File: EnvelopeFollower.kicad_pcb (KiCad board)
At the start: 2 copper layers, 177.9 x 87.9 mm, 87 parts, among them J1 RTip, J10 IN, J11 GND, J12 GND, J13 SW1B, J14 OUT, J15 DTIP, J16 DSW, J17 GND, J18 ITIP, J19 ISLV, J20 SW1C, J3 +9v, J4 GND, J5 SEND, J6 RSLV, J7 GND, J8 GND, J9 SW1A, SW1 Moog, SW2 BANDWIDTH, SW3 MODE, U1 TL074, U2 LM1458, U3 VTL5C, U4 VTL5C

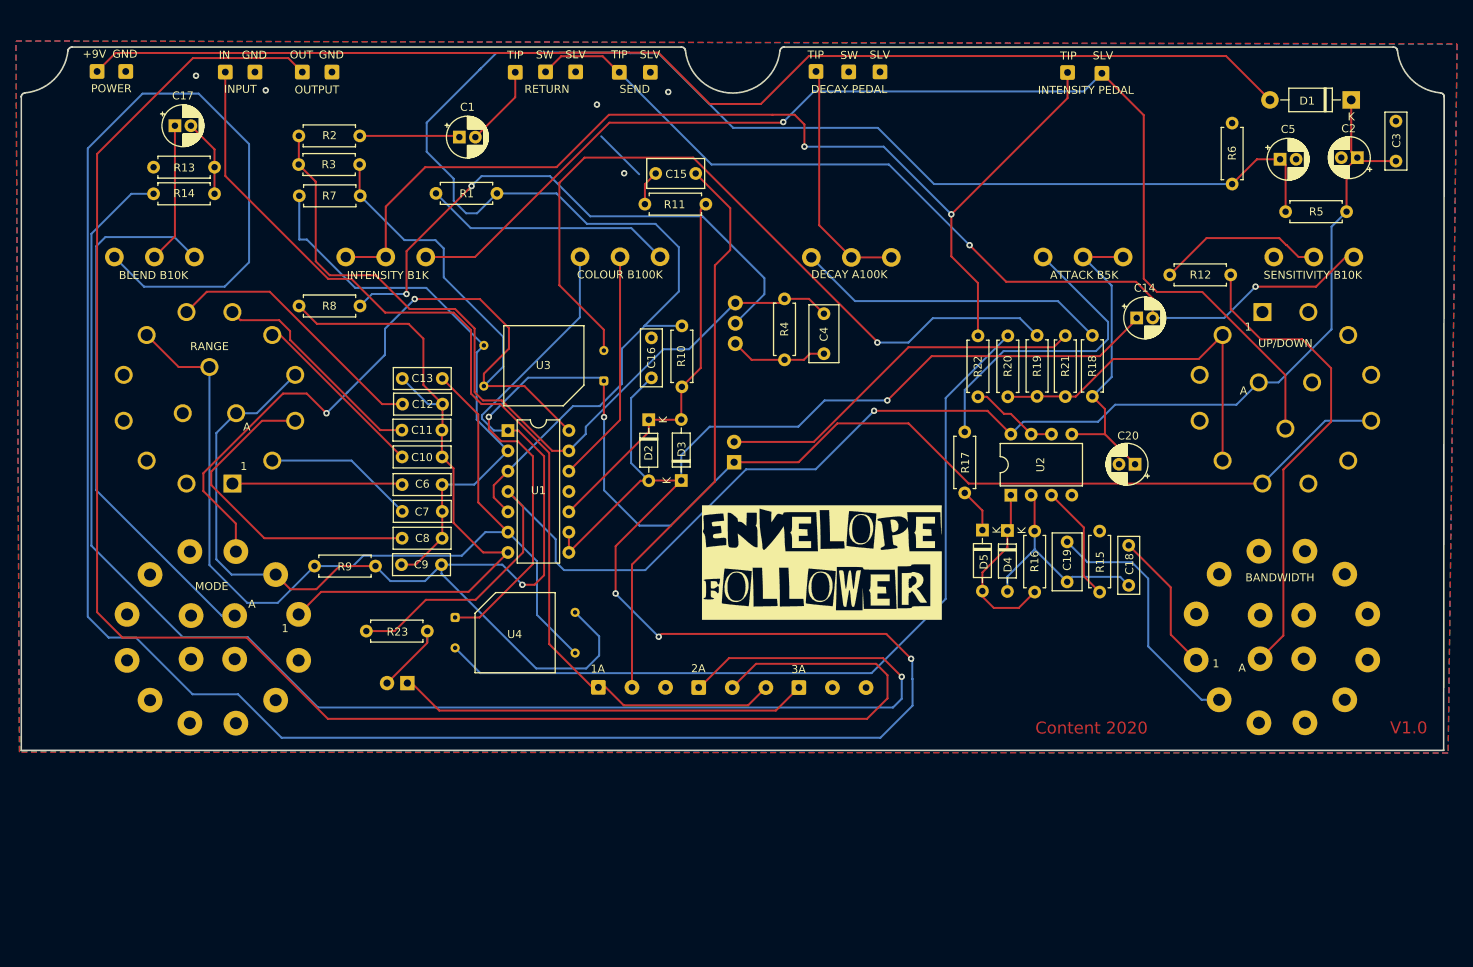
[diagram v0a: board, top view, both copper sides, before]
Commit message: V2.00 provisionaly completed
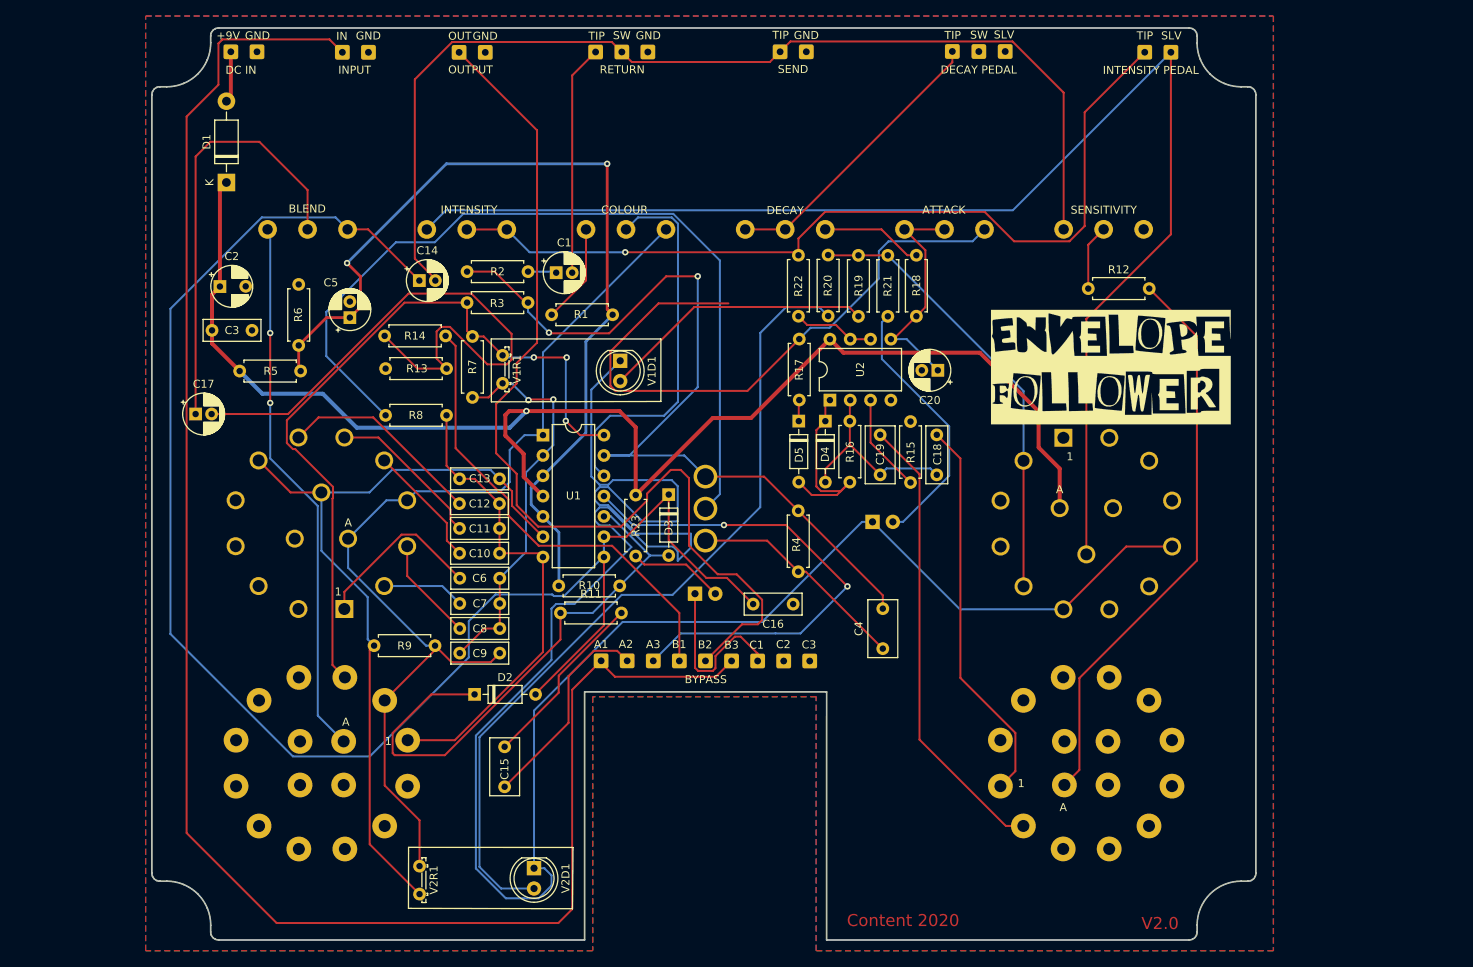
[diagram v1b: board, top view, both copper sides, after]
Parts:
- removed U3, U4: VTL5C, OptoDevice:PerkinElmer_VTL5C
- added J2: 1A3, Connector_Wire:SolderWire-0.25sqmm_1x01_D0.65mm_OD1.7mm, F.Cu at (125.7, 117.4)
- added J21: 1B2, Connector_Wire:SolderWire-0.25sqmm_1x01_D0.65mm_OD1.7mm, F.Cu at (132.2, 117.4)
- added J22: 1B1, Connector_Wire:SolderWire-0.25sqmm_1x01_D0.65mm_OD1.7mm, F.Cu at (128.9, 117.4)
- added J23: 1C1, Connector_Wire:SolderWire-0.25sqmm_1x01_D0.65mm_OD1.7mm, F.Cu at (138.7, 117.5)
- added J24: 1C2, Connector_Wire:SolderWire-0.25sqmm_1x01_D0.65mm_OD1.7mm, F.Cu at (142.0, 117.5)
- added J25: 1C3, Connector_Wire:SolderWire-0.25sqmm_1x01_D0.65mm_OD1.7mm, F.Cu at (145.2, 117.5)
- added V1D1: D_Photo, MyLibrary:LED_D5.0mm, F.Cu at (121.6, 79.9)
- added V1R1: D_LDR, MyLibrary:R_LDR_5.2x5.2mm_P3.5mm_Horizontal, F.Cu at (106.8, 79.2)
- added V2D1: D_Photo, MyLibrary:LED_D5.0mm, F.Cu at (110.8, 143.4)
- added V2R1: D_LDR, MyLibrary:R_LDR_5.2x5.2mm_P3.5mm_Horizontal, F.Cu at (96.5, 143.1)
- C2: footprint Capacitor_THT:CP_Radial_D5.0mm_P2.00mm -> MyLibrary:CP_Radial_D5.0mm_PWideForPower
- J13: value SW1B -> 1A1; footprint Connector_Wire:SolderWire-0.25sqmm_1x03_P4.2mm_D0.65mm_OD1.7mm -> Connector_Wire:SolderWire-0.25sqmm_1x01_D0.65mm_OD1.7mm
- J20: value SW1C -> 1B3; footprint Connector_Wire:SolderWire-0.25sqmm_1x03_P4.2mm_D0.65mm_OD1.7mm -> Connector_Wire:SolderWire-0.25sqmm_1x01_D0.65mm_OD1.7mm
- J9: value SW1A -> 1A2; footprint Connector_Wire:SolderWire-0.25sqmm_1x03_P4.2mm_D0.65mm_OD1.7mm -> Connector_Wire:SolderWire-0.25sqmm_1x01_D0.65mm_OD1.7mm
- R22: value 1M8 -> 330r
- SW1: footprint Switches:SWITCH_SPDT_PTH_11.6X4.0MM -> MyLibrary:SWITCH_SPDT_PTH_12.9X6.9MM
- moved C3 149.5 mm to (70.5, 76.1), turned to 0 degrees
- moved C2 142.6 mm to (72.0, 70.6), turned to 0 degrees
- moved D1 141.0 mm to (72.3, 57.6), turned to 90 degrees
- moved R5 139.8 mm to (74.0, 81.2), turned to 0 degrees
- moved R6 118.4 mm to (81.4, 78.0)
- moved C5 118.0 mm to (87.8, 74.5), turned to 90 degrees
- moved C14 89.8 mm to (96.4, 69.9)
- moved C15 80.3 mm to (107.1, 133.2), turned to 90 degrees
- moved R11 54.2 mm to (114.1, 111.5), turned to 0 degrees
- moved G*** 43.6 mm to (182.9, 80.7)
- moved D2 40.7 mm to (103.3, 121.6), turned to 0 degrees
- moved R14 40.6 mm to (99.7, 76.8), turned to 180 degrees
- moved G*** 39.1 mm to (178.0, 77.5)
- moved R13 38.4 mm to (99.8, 80.9)
- moved C16 37.7 mm to (143.2, 110.3), turned to 180 degrees
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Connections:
- net /Vact1-4 renamed Net-(C6-Pad2)
- J13 pad 1: Net-(J13-Pad1) -> Net-(J10-Pad1)
- J14 pad 1: Net-(J13-Pad2) -> Net-(J14-Pad1)
- J20 pad 1: Net-(D7-Pad1) -> Net-(J10-Pad1)
- J9 pad 1: Net-(J10-Pad1) -> Net-(C15-Pad1)
- R14 pad 1: Net-(J13-Pad1) -> Net-(J22-Pad1)
- R19 pad 2: /Vact1-2 -> Net-(R19-Pad2)
- R20 pad 2: /Vact2-2 -> Net-(R20-Pad2)
- RV1 pad 1: /Mode2 -> Net-(R1-Pad1)
- RV1 pad 3: Net-(R1-Pad1) -> /Mode2
- RV2 pad 1: GND -> Net-(C14-Pad2)
- RV2 pad 3: Net-(C14-Pad2) -> GND
- RV3 pad 1: Net-(C14-Pad1) -> /ModeA
- RV3 pad 3: /ModeA -> Net-(C14-Pad1)
- RV4 pad 1: Net-(R17-Pad2) -> Net-(C20-Pad1)
- RV4 pad 3: Net-(C20-Pad1) -> Net-(R17-Pad2)
- RV5 pad 1: Net-(R18-Pad2) -> Net-(J15-Pad1)
- RV5 pad 3: Net-(J15-Pad1) -> Net-(R18-Pad2)
- RV6 pad 1: Net-(J18-Pad1) -> /UDB
- RV6 pad 3: /UDB -> Net-(J18-Pad1)
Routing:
- net Net-(J13-Pad2): track 218.1 -> 0.00 mm
- net Net-(J13-Pad1): track 189.6 -> 0.00 mm, vias 1 -> 0
- net Net-(C14-Pad1): track 396.1 -> 209.0 mm, vias 4 -> 0
- net +9VA: track 155.0 -> 7.19 mm
- net Net-(J14-Pad1): track 0.00 -> 122.5 mm
- net VCC: track 219.3 -> 115.6 mm, vias 0 -> 2
- net Net-(R20-Pad2): track 0.00 -> 103.2 mm
- net /Vact2-2: track 102.6 -> 0.00 mm
- net /Vact1-2: track 96.1 -> 0.00 mm, vias 1 -> 0
- net Net-(J10-Pad1): track 127.5 -> 220.9 mm
- net /UD6: track 174.0 -> 266.5 mm, vias 2 -> 0
- net Net-(C17-Pad2): track 9.73 -> 75.4 mm
- net GND: track 0.00 -> 63.2 mm, vias 5 -> 2
- net Net-(J22-Pad1): track 0.00 -> 58.2 mm
- net Net-(C15-Pad1): track 71.1 -> 26.3 mm
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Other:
- board size 177.9 x 87.9 mm -> 138 x 114 mm
- net class Power added: clearance 0.5, trace_width 0.5, via_dia 0.8, via_drill 0.4
- net class VCC added: clearance 0.35, trace_width 0.35, via_dia 0.8, via_drill 0.4
- board text added: "A1"
- board text added: "A2"
- board text added: "A3"
- board text added: "ATTACK"
- board text added: "B1"
- board text added: "B2"
- board text added: "B3"
- board text added: "BLEND"
- board text added: "BYPASS"
- board text added: "C1"
- board text added: "C2"
- board text added: "C3"
- board text added: "COLOUR"
- board text added: "DC IN"
- board text added: "DECAY"
- board text added: "INTENSITY"
- board text added: "SENSITIVITY"
- board text added: "V2.0"
- board text removed: "1A"
- board text removed: "2A"
- board text removed: "3A"
- board text removed: "ATTACK B5K"
- board text removed: "BANDWIDTH"
- board text removed: "BLEND B10K"
- board text removed: "COLOUR B100K"
- board text removed: "DECAY A100K"
- board text removed: "INTENSITY B1K"
- board text removed: "MODE"
- board text removed: "POWER"
- board text removed: "RANGE"
- board text removed: "SENSITIVITY B10K"
- board text removed: "UP/DOWN"
- board text removed: "V1.0"
